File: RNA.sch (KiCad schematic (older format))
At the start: 89 parts, among them J1 USB_B_Micro, J2 SM04B-SRSS-TB(LF)(SN), J3 AudioJack4, J4 Conn_01x06, SW1 SW_SPST, SW10 CPG135001S30, SW11 CPG135001S30, SW12 CPG135001S30, SW13 CPG135001S30, SW14 CPG135001S30, SW15 CPG135001S30, SW16 CPG135001S30, SW17 CPG135001S30, SW18 CPG135001S30, SW19 CPG135001S30, SW2 SW_Push, SW20 CPG135001S30, SW21 CPG135001S30, SW22 CPG135001S30, SW23 CPG135001S30, SW24 CPG135001S30, SW25 CPG135001S30, SW26 CPG135001S30, SW27 CPG135001S30, SW28 CPG135001S30, SW29 CPG135001S30, SW3 CPG135001S30, SW30 CPG135001S30, SW31 CPG135001S30, SW32 CPG135001S30, SW33 CPG135001S30, SW34 CPG135001S30, SW4 CPG135001S30, SW5 CPG135001S30, SW6 CPG135001S30, SW7 CPG135001S30, SW8 CPG135001S30, SW9 CPG135001S30, U1 STM32F072C8Tx, U2 PRTR5V0U2X, U3 MCP1703A-3302_SOT23

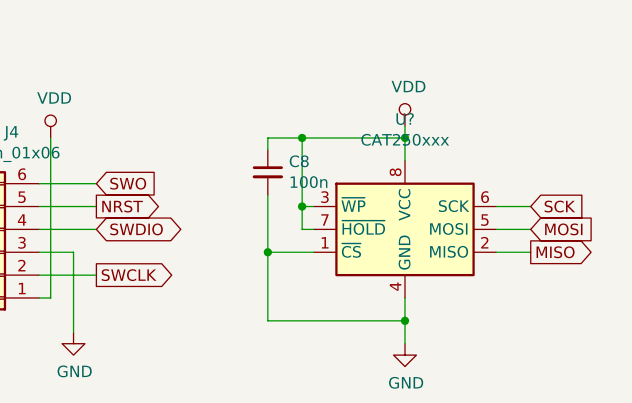
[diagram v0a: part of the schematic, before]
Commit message: more routing
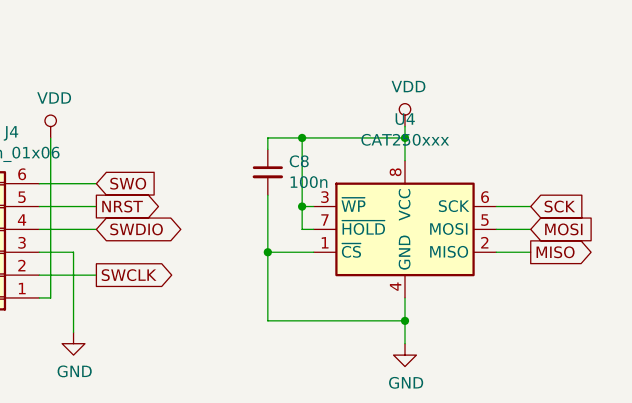
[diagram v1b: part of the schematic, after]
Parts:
- C1, C2, C3, C4, C5: footprint Capacitor_SMD:C_0603_1608Metric -> Capacitor_SMD:C_0402_1005Metric
- U4: renamed from U?; footprint (none) -> Package_SO:SOIC-8_3.9x4.9mm_P1.27mm
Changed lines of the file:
@@
 F 0 "C1" H 2892 996 50  0000 L CNN
 F 1 "100n" H 2892 905 50  0000 L CNN
-F 2 "Capacitor_SMD:C_0603_1608Metric" H 2800 950 50  0001 C CNN
+F 2 "Capacitor_SMD:C_0402_1005Metric" H 2800 950 50  0001 C CNN
 F 3 "~" H 2800 950 50  0001 C CNN
 	1    2800 950
@@
 F 0 "C2" H 3092 996 50  0000 L CNN
 F 1 "100n" H 3092 905 50  0000 L CNN
-F 2 "Capacitor_SMD:C_0603_1608Metric" H 3000 950 50  0001 C CNN
+F 2 "Capacitor_SMD:C_0402_1005Metric" H 3000 950 50  0001 C CNN
 F 3 "~" H 3000 950 50  0001 C CNN
 	1    3000 950
@@
 F 0 "C3" H 3292 996 50  0000 L CNN
 F 1 "100n" H 3292 905 50  0000 L CNN
-F 2 "Capacitor_SMD:C_0603_1608Metric" H 3200 950 50  0001 C CNN
+F 2 "Capacitor_SMD:C_0402_1005Metric" H 3200 950 50  0001 C CNN
 F 3 "~" H 3200 950 50  0001 C CNN
 	1    3200 950
@@
 F 0 "C4" H 3692 996 50  0000 L CNN
 F 1 "100n" H 3692 905 50  0000 L CNN
-F 2 "Capacitor_SMD:C_0603_1608Metric" H 3600 950 50  0001 C CNN
+F 2 "Capacitor_SMD:C_0402_1005Metric" H 3600 950 50  0001 C CNN
 F 3 "~" H 3600 950 50  0001 C CNN
 	1    3600 950
@@
 F 0 "C5" H 4642 1496 50  0000 L CNN
 F 1 "100u" H 4642 1405 50  0000 L CNN
-F 2 "Capacitor_SMD:C_0603_1608Metric" H 4550 1450 50  0001 C CNN
+F 2 "Capacitor_SMD:C_0402_1005Metric" H 4550 1450 50  0001 C CNN
 F 3 "~" H 4550 1450 50  0001 C CNN
 	1    4550 1450
@@
 	2350 2900 2500 2900
 $Comp
-L Memory_EEPROM:CAT250xxx U?
+L Memory_EEPROM:CAT250xxx U4
 U 1 1 5D17739A
 P 10000 1350
-F 0 "U?" H 10000 1831 50  0000 C CNN
+F 0 "U4" H 10000 1831 50  0000 C CNN
 F 1 "CAT250xxx" H 10000 1740 50  0000 C CNN
-F 2 "" H 10000 1350 50  0001 C CNN
+F 2 "Package_SO:SOIC-8_3.9x4.9mm_P1.27mm" H 10000 1350 50  0001 C CNN
 F 3 "http://www.onsemi.com/PowerSolutions/product.do?id=CAT25040" H 10000 1350 50  0001 C CNN
 	1    10000 1350
